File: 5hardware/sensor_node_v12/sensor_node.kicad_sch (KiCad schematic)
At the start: 38 parts, among them J1 Conn_01x08_Socket, J2 Conn_01x08_Socket, Q2 AO3401A, Q3 MMBT5551L, Q4 AO3401A, SW2 SW_Push, SW4 SW_Reed, SW5 SW_Push, SW6 SW_Push, U1 ESP-12F, U12 APDS-9960, U13 SHT31-DIS, U17 BH1750FVI-TR, U2 2N7002DW, U4 CH32V003F4P6, U7 XC6206PxxxMR, U8 TPL5110

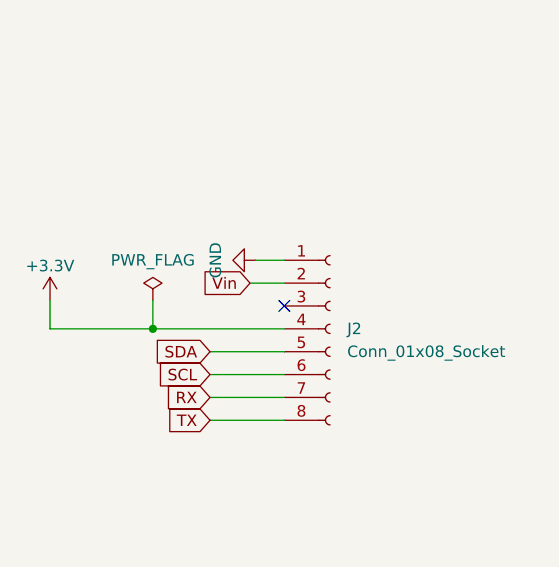
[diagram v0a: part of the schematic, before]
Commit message: did some works.
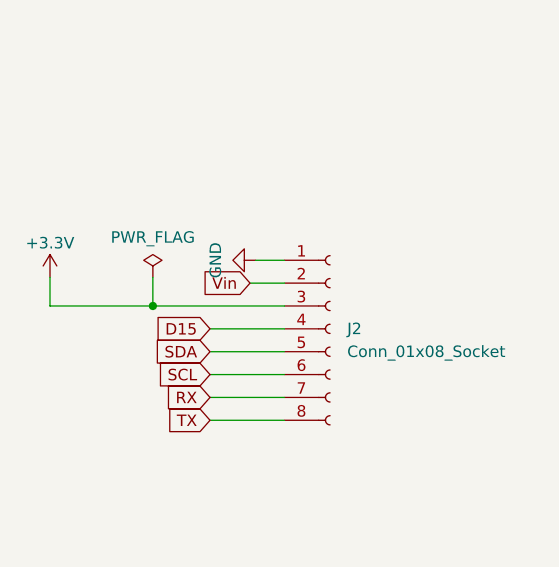
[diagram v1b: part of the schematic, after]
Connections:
- net +3.3V: now also J2.3 (Pin_3); no longer J2.4 (Pin_4)
- net D15: now also J2.4 (Pin_4)
- no-connect marks 24 -> 23
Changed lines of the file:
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@@
   (junction (at 76.2 108.585) (diameter 0) (color 0 0 0 0)
   )
-  (junction (at 62.865 192.405) (diameter 0) (color 0 0 0 0)
+  (junction (at 62.865 189.865) (diameter 0) (color 0 0 0 0)
   )
   (junction (at 317.5 95.885) (diameter 0) (color 0 0 0 0)
@@
   (no_connect (at 240.665 184.15))
   (no_connect (at 243.205 184.15))
-  (no_connect (at 77.47 189.865))
   (no_connect (at 149.86 203.835))
   (no_connect (at 256.54 226.06))
@@
   (no_connect (at 226.06 236.22))
   (no_connect (at 245.745 184.15))
-  (wire (pts (xy 51.435 189.23) (xy 51.435 192.405))
+  (wire (pts (xy 51.435 186.69) (xy 51.435 189.865))
     (stroke (width 0) (type default))
   )
@@
     (stroke (width 0) (type default))
   )
+  (wire (pts (xy 77.47 192.405) (xy 69.215 192.405))
+    (stroke (width 0) (type default))
+  )
   (wire (pts (xy 74.295 184.785) (xy 77.47 184.785))
     (stroke (width 0) (type default))
@@
     (stroke (width 0) (type default))
   )
-  (wire (pts (xy 62.865 192.405) (xy 77.47 192.405))
+  (wire (pts (xy 62.865 189.865) (xy 77.47 189.865))
     (stroke (width 0) (type default))
   )
@@
     (stroke (width 0) (type default))
   )
-  (wire (pts (xy 62.865 189.23) (xy 62.865 192.405))
+  (wire (pts (xy 62.865 186.69) (xy 62.865 189.865))
     (stroke (width 0) (type default))
   )
@@
     (stroke (width 0) (type default))
   )
-  (wire (pts (xy 62.865 192.405) (xy 51.435 192.405))
+  (wire (pts (xy 62.865 189.865) (xy 51.435 189.865))
     (stroke (width 0) (type default))
   )
@@
     (effects (font (size 1.27 1.27)) (justify right))
     (property "Intersheetrefs" "${INTERSHEET_REFS}" (at 135.8379 193.675 0)
+      (effects (font (size 1.27 1.27)) (justify right) hide)
+    )
+  )
+  (global_label "D15" (shape input) (at 69.215 192.405 180) (fields_autoplaced)
+    (effects (font (size 1.27 1.27)) (justify right))
+    (property "Intersheetrefs" "${INTERSHEET_REFS}" (at 62.5408 192.405 0)
       (effects (font (size 1.27 1.27)) (justify right) hide)
     )
@@
     )
   )
-  (symbol (lib_id "power:PWR_FLAG") (at 62.865 189.23 0) (mirror y) (unit 1)
-    (in_bom yes) (on_board yes) (dnp no)
-    (property "Reference" "#FLG04" (at 62.865 187.325 0)
-      (effects (font (size 1.27 1.27)) hide)
-    )
-    (property "Value" "PWR_FLAG" (at 62.865 184.785 0)
-      (effects (font (size 1.27 1.27)))
-    )
-    (property "Footprint" "" (at 62.865 189.23 0)
-      (effects (font (size 1.27 1.27)) hide)
-    )
-    (property "Datasheet" "~" (at 62.865 189.23 0)
+  (symbol (lib_id "power:PWR_FLAG") (at 62.865 186.69 0) (mirror y) (unit 1)
+    (in_bom yes) (on_board yes) (dnp no)
+    (property "Reference" "#FLG04" (at 62.865 184.785 0)
+      (effects (font (size 1.27 1.27)) hide)
+    )
+    (property "Value" "PWR_FLAG" (at 62.865 182.245 0)
+      (effects (font (size 1.27 1.27)))
+    )
+    (property "Footprint" "" (at 62.865 186.69 0)
+      (effects (font (size 1.27 1.27)) hide)
+    )
+    (property "Datasheet" "~" (at 62.865 186.69 0)
       (effects (font (size 1.27 1.27)) hide)
     )
@@
     )
   )
-  (symbol (lib_id "power:+3.3V") (at 51.435 189.23 0) (mirror y) (unit 1)
-    (in_bom yes) (on_board yes) (dnp no)
-    (property "Reference" "#PWR010" (at 51.435 193.04 0)
-      (effects (font (size 1.27 1.27)) hide)
-    )
-    (property "Value" "+3.3V" (at 51.435 185.42 0)
-      (effects (font (size 1.27 1.27)))
-    )
-    (property "Footprint" "" (at 51.435 189.23 0)
-      (effects (font (size 1.27 1.27)) hide)
-    )
-    (property "Datasheet" "" (at 51.435 189.23 0)
-      (effects (font (size 1.27 1.27)) hide)
-    )
+  (symbol (lib_id "power:+3.3V") (at 51.435 186.69 0) (mirror y) (unit 1)
+    (in_bom yes) (on_board yes) (dnp no)
+    (property "Reference" "#PWR010" (at 51.435 190.5 0)
+      (effects (font (size 1.27 1.27)) hide)
+    )
+    (property "Value" "+3.3V" (at 51.435 182.88 0)
+      (effects (font (size 1.27 1.27)))
+    )
+    (property "Footprint" "" (at 51.435 186.69 0)
+      (effects (font (size 1.27 1.27)) hide)
+    )
+    (property "Datasheet" "" (at 51.435 186.69 0)
+      (effects (font (size 1.27 1.27)) hide)
+    )
